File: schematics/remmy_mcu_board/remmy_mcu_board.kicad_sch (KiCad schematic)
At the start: 25 parts, among them J1 AVR-JTAG-10, J2 Conn_02x05_Counter_Clockwise, J3 Conn_01x03_Pin, Q1 BSS138, SW1 RotaryEncoder, SW2 SW_Push, SW3 SW_Push, SW4 SW_Push, U1 NX3225SA-16, U2 ATmega32U4-M, U3 Kailh GM 8.0, U4 Kailh GM 8.0

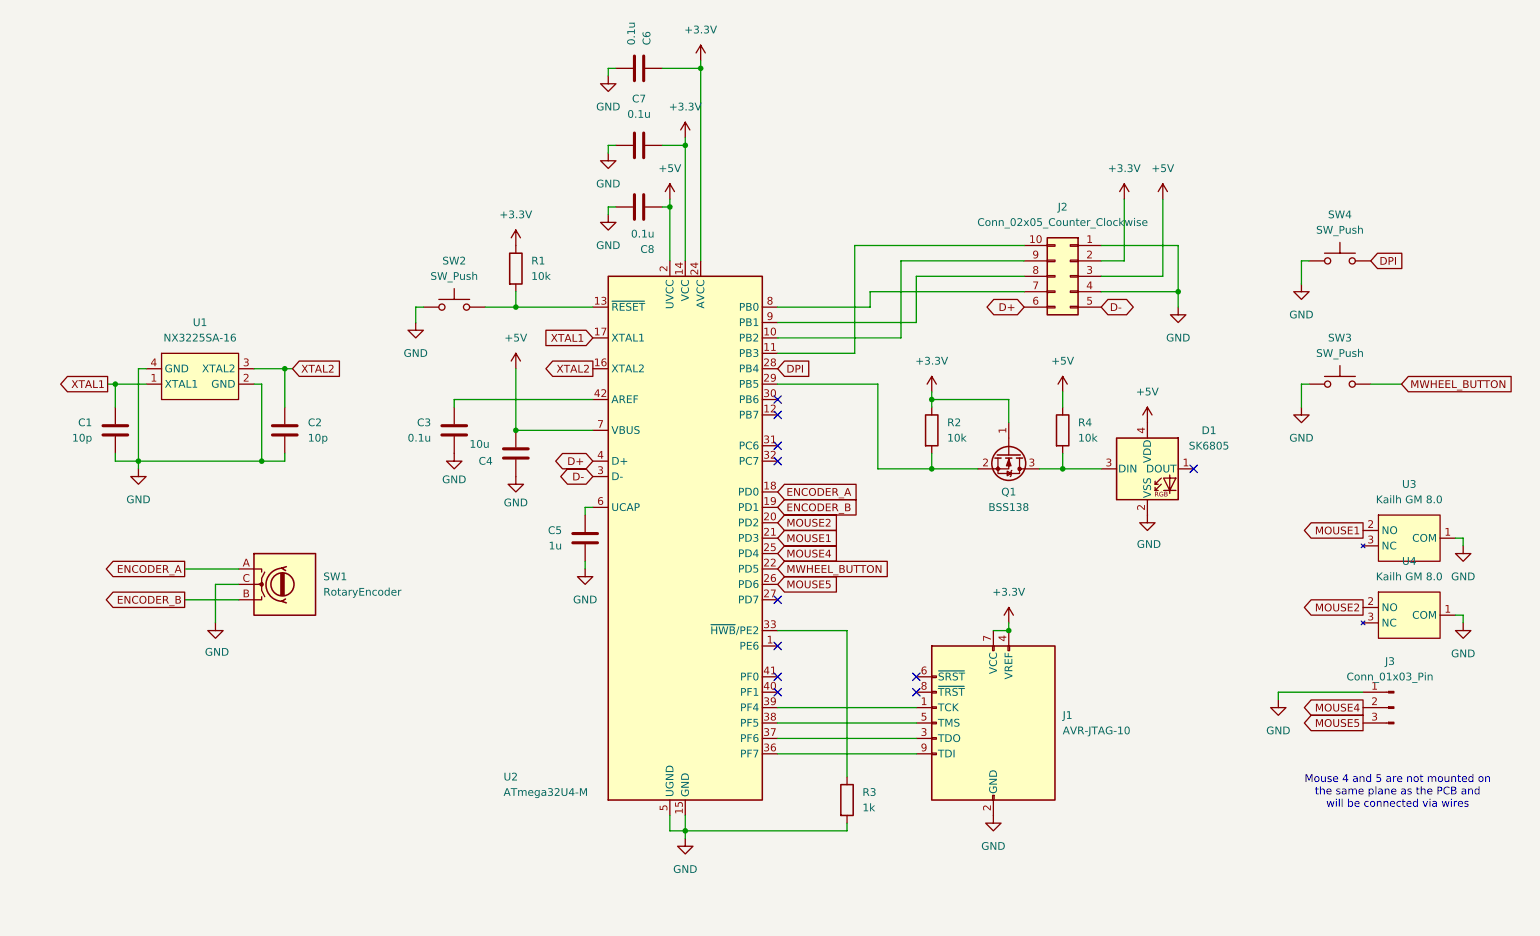
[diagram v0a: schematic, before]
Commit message: added images
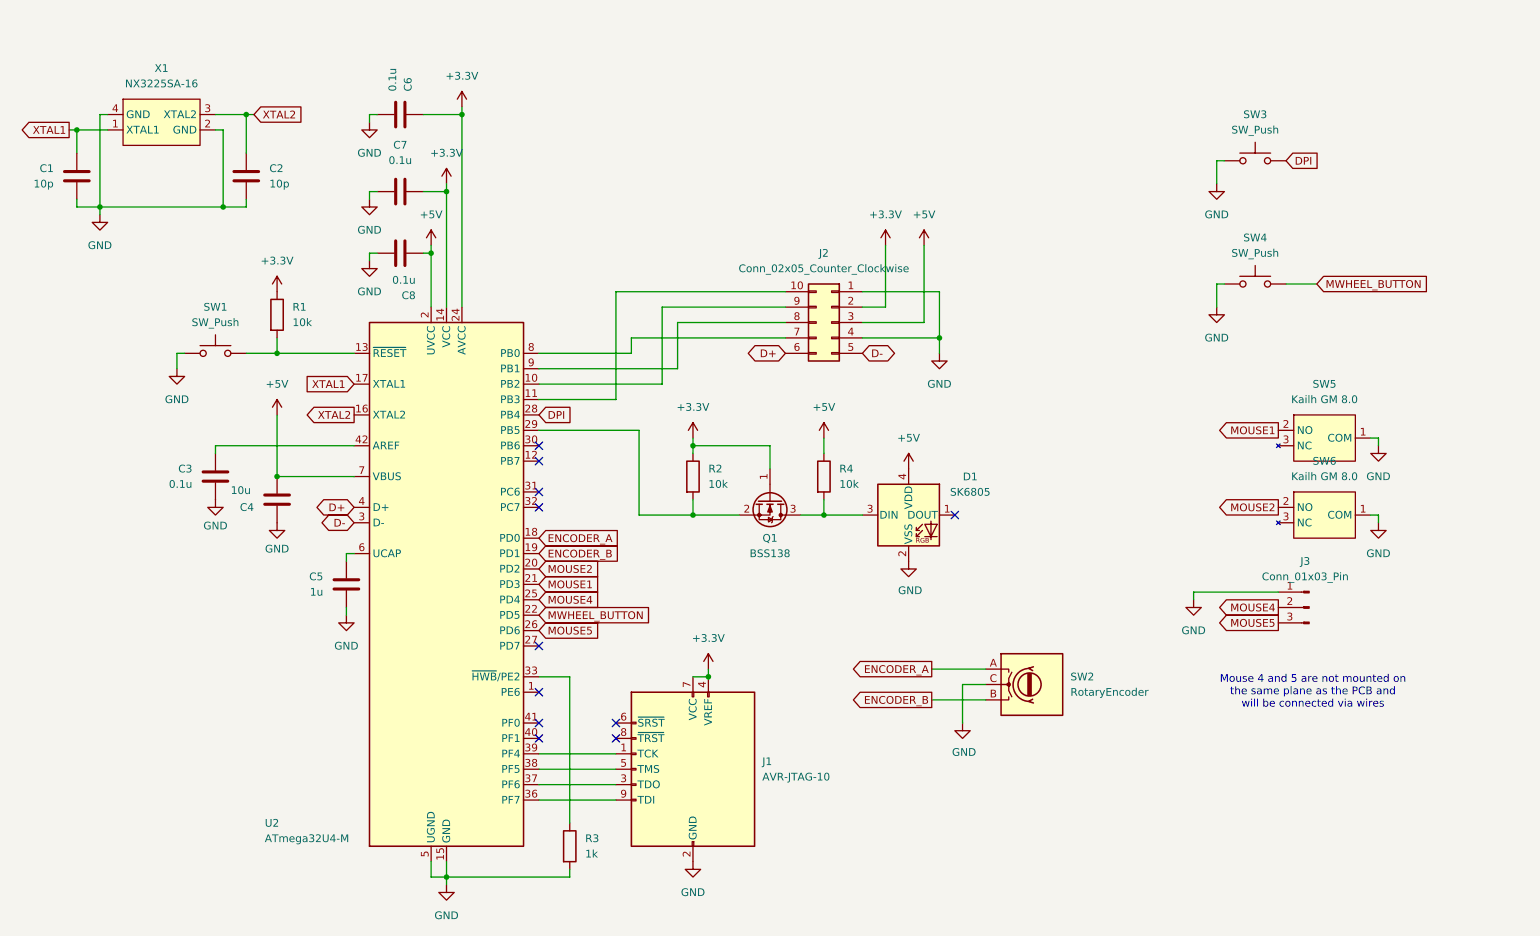
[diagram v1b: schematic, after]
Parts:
- renumbered SW2 to SW1, SW1 to SW2, SW4 to SW3, SW3 to SW4, U3 to SW5, U4 to SW6, U1 to X1
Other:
- title: (none) -> Remmy A
- moved on the sheet: C1, C2, C3, C4, C5, C6, C7, C8, D1, J1, J2, J3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
